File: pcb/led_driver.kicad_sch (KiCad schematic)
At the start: 69 parts, among them J1 48V IN, J2 LED, J3 12V IN, J4 INTERLOCK, Q1 STP30NF10, SW3 ARM, U1 MIC4427, U2 74HC74, U3 74HC08, U4 LM393, U5 L7805

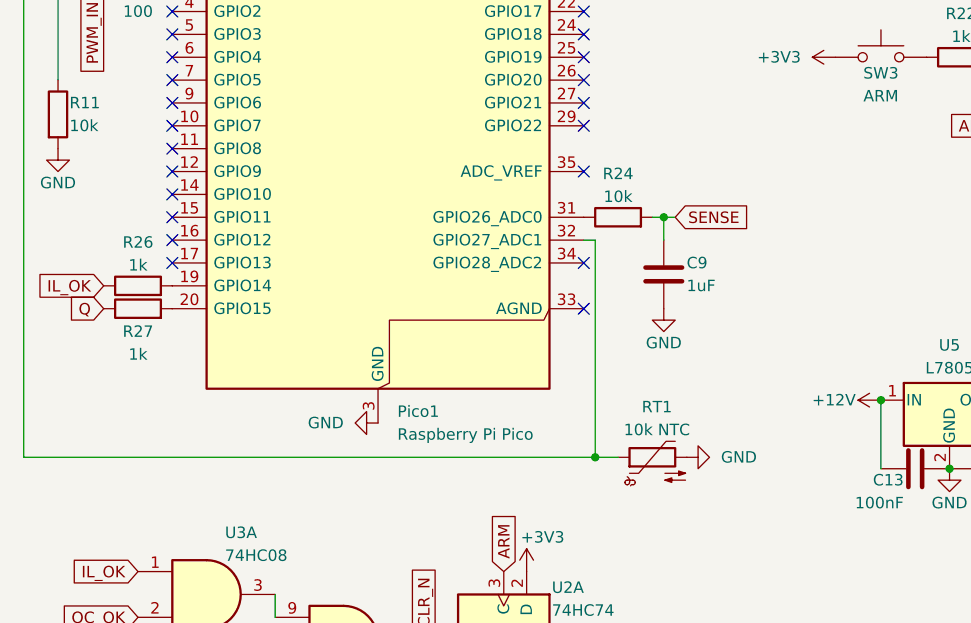
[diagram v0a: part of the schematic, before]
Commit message: First revision
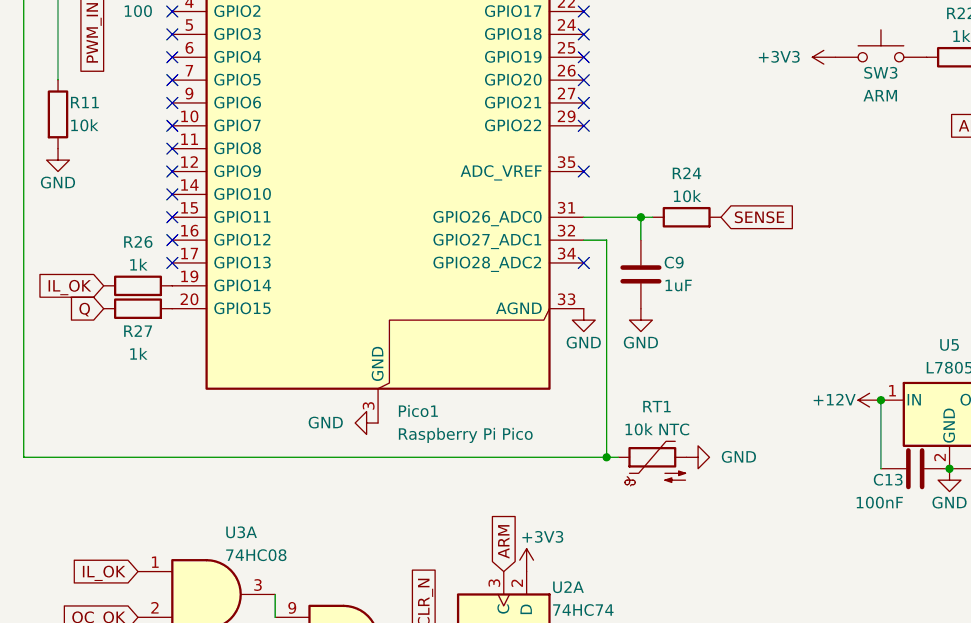
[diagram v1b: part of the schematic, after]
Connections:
- net GND: now also Pico1.33 (AGND)
- net SENSE: no longer C9.1
- net at Pico1.31 (GPIO26_ADC0), R24.1: now also C9.1
- no-connect marks 29 -> 28
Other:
- moved on the sheet: C9, R24
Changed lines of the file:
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@@
 		(title "Fast-Switching LED Driver")
 		(date "2026-09-28")
-		(rev "0")
+		(rev "1")
 	)
 	(text "R2\n4 x 0.39"
@@
 	)
 	(junction
-		(at 111.76 83.82)
+		(at 109.22 83.82)
 		(diameter 0)
 		(color 0 0 0 0)
@@
 	)
 	(junction
-		(at 104.14 110.49)
+		(at 105.41 110.49)
 		(diameter 0)
 		(color 0 0 0 0)
@@
 	)
 	(no_connect
-		(at 102.87 93.98)
-	)
-	(no_connect
 		(at 57.15 81.28)
 	)
@@
 	(wire
 		(pts
-			(xy 102.87 86.36) (xy 104.14 86.36)
+			(xy 102.87 86.36) (xy 105.41 86.36)
 		)
 		(stroke
@@
 	(wire
 		(pts
+			(xy 109.22 83.82) (xy 109.22 86.36)
+		)
+		(stroke
+			(width 0)
+			(type default)
+		)
+	)
+	(wire
+		(pts
 			(xy 203.2 66.04) (xy 199.39 66.04)
 		)
@@
 	(wire
 		(pts
-			(xy 104.14 86.36) (xy 104.14 110.49)
+			(xy 105.41 86.36) (xy 105.41 110.49)
 		)
 		(stroke
@@
 	(wire
 		(pts
-			(xy 111.76 86.36) (xy 111.76 83.82)
-		)
-		(stroke
-			(width 0)
-			(type default)
-		)
-	)
-	(wire
-		(pts
 			(xy 231.14 31.75) (xy 236.22 31.75)
 		)
@@
 	(wire
 		(pts
-			(xy 104.14 110.49) (xy 106.68 110.49)
-		)
-		(stroke
-			(width 0)
-			(type default)
-		)
-	)
-	(wire
-		(pts
 			(xy 57.15 21.59) (xy 85.09 21.59)
 		)
@@
 	(wire
 		(pts
-			(xy 113.03 83.82) (xy 111.76 83.82)
-		)
-		(stroke
-			(width 0)
-			(type default)
-		)
-	)
-	(wire
-		(pts
 			(xy 207.01 137.16) (xy 217.17 137.16)
 		)
@@
 	(wire
 		(pts
-			(xy 111.76 83.82) (xy 110.49 83.82)
+			(xy 229.87 36.83) (xy 231.14 36.83)
 		)
 		(stroke
@@
 	(wire
 		(pts
-			(xy 229.87 36.83) (xy 231.14 36.83)
+			(xy 85.09 21.59) (xy 85.09 33.02)
 		)
 		(stroke
@@
 	(wire
 		(pts
-			(xy 85.09 21.59) (xy 85.09 33.02)
+			(xy 40.64 21.59) (xy 40.64 110.49)
 		)
 		(stroke
@@
 	(wire
 		(pts
-			(xy 40.64 21.59) (xy 40.64 110.49)
+			(xy 40.64 110.49) (xy 106.68 110.49)
 		)
 		(stroke
@@
 	(wire
 		(pts
-			(xy 40.64 110.49) (xy 104.14 110.49)
+			(xy 243.84 66.04) (xy 243.84 57.15)
 		)
 		(stroke
@@
 	(wire
 		(pts
-			(xy 243.84 66.04) (xy 243.84 57.15)
+			(xy 148.59 46.99) (xy 151.13 46.99)
 		)
 		(stroke
@@
 	(wire
 		(pts
-			(xy 148.59 46.99) (xy 151.13 46.99)
+			(xy 199.39 36.83) (xy 196.85 36.83)
 		)
 		(stroke
@@
 	(wire
 		(pts
-			(xy 199.39 36.83) (xy 196.85 36.83)
+			(xy 195.58 137.16) (xy 200.66 137.16)
 		)
 		(stroke
@@
 	(wire
 		(pts
-			(xy 195.58 137.16) (xy 200.66 137.16)
+			(xy 102.87 83.82) (xy 110.49 83.82)
 		)
 		(stroke
@@
 	(global_label "SENSE"
 		(shape input)
-		(at 113.03 83.82 0)
+		(at 118.11 83.82 0)
 		(fields_autoplaced yes)
 		(effects
@@
 		)
 		(property "Intersheetrefs" "${INTERSHEET_REFS}"
-			(at 122.0627 83.82 0)
+			(at 127.1427 83.82 0)
 			(hide yes)
 			(show_name no)
@@
 	(symbol
 		(lib_id "Device:C")
-		(at 111.76 90.17 0)
+		(at 109.22 90.17 0)
 		(unit 1)
 		(body_style 1)
@@
 		(dnp no)
 		(property "Reference" "C9"
-			(at 114.3 88.9 0)
+			(at 111.76 88.9 0)
 			(show_name no)
 			(do_not_autoplace no)
@@
 		)
 		(property "Value" "1uF"
-			(at 114.3 91.44 0)
+			(at 111.76 91.44 0)
 			(show_name no)
 			(do_not_autoplace no)
@@
 		)
 		(property "Footprint" "Capacitor_THT:C_Rect_L7.2mm_W4.5mm_P5.00mm_FKS2_FKP2_MKS2_MKP2"
-			(at 112.7252 93.98 0)
+			(at 110.1852 93.98 0)
 			(hide yes)
 			(show_name no)
@@
 		)
 		(property "Datasheet" ""
-			(at 111.76 90.17 0)
+			(at 109.22 90.17 0)
 			(hide yes)
 			(show_name no)
@@
 		)
 		(property "Description" "Unpolarized capacitor"
-			(at 111.76 90.17 0)
+			(at 109.22 90.17 0)
 			(hide yes)
 			(show_name no)
@@
 	(symbol
 		(lib_id "Device:R")
-		(at 106.68 83.82 90)
+		(at 114.3 83.82 90)
 		(unit 1)
 		(body_style 1)
@@
 		(dnp no)
 		(property "Reference" "R24"
-			(at 106.68 78.994 90)
+			(at 114.3 78.994 90)
 			(show_name no)
 			(do_not_autoplace no)
@@
 		)
 		(property "Value" "10k"
-			(at 106.68 81.534 90)
+			(at 114.3 81.534 90)
 			(show_name no)
 			(do_not_autoplace no)
@@
 		)
 		(property "Footprint" "Resistor_THT:R_Axial_DIN0207_L6.3mm_D2.5mm_P10.16mm_Horizontal"
-			(at 106.68 85.598 90)
+			(at 114.3 85.598 90)
 			(hide yes)
 			(show_name no)
@@
 		)
 		(property "Datasheet" ""
-			(at 106.68 83.82 0)
+			(at 114.3 83.82 0)
 			(hide yes)
 			(show_name no)
@@
 		)
 		(property "Description" "Resistor"
-			(at 106.68 83.82 0)
+			(at 114.3 83.82 0)
 			(hide yes)
 			(show_name no)
@@
 	)
 	(symbol
+		(lib_id "power:GND")
+		(at 102.87 93.98 0)
+		(unit 1)
+		(body_style 1)
+		(exclude_from_sim no)
+		(in_bom yes)
+		(on_board yes)
+		(in_pos_files yes)
+		(dnp no)
+		(property "Reference" "#PWR035"
+			(at 102.87 100.33 0)
+			(hide yes)
+			(show_name no)
+			(do_not_autoplace no)
+			(effects
+				(font
+					(size 1.27 1.27)
+				)
+			)
+		)
+		(property "Value" "GND"
+			(at 102.87 97.79 0)
+			(show_name no)
+			(do_not_autoplace no)
+			(effects
+				(font
+					(size 1.27 1.27)
+				)
+			)
+		)
+		(property "Footprint" ""
+			(at 102.87 93.98 0)
+			(hide yes)
+			(show_name no)
+			(do_not_autoplace no)
+			(effects
+				(font
+					(size 1.27 1.27)
+				)
+			)
+		)
+		(property "Datasheet" ""
+			(at 102.87 93.98 0)
+			(hide yes)
+			(show_name no)
+			(do_not_autoplace no)
+			(effects
+				(font
+					(size 1.27 1.27)
+				)
+			)
+		)
+		(property "Description" "Power symbol creates a global label with name \"GND\" , ground"
+			(at 102.87 93.98 0)
+			(hide yes)
+			(show_name no)
+			(do_not_autoplace no)
+			(effects
+				(font
+					(size 1.27 1.27)
+				)
+			)
+		)
+		(pin "1"
+		)
+		(instances
+			(project "led_driver"
+				(path "/517fb8ba-efa2-4ff9-8737-3053492b2e56"
+					(reference "#PWR035")
+					(unit 1)
+				)
+			)
+		)
+	)
+	(symbol
 		(lib_id "Connector:Screw_Terminal_01x02")
 		(at 259.08 152.4 270)
@@
 	(symbol
 		(lib_id "power:GND")
-		(at 111.76 93.98 0)
+		(at 109.22 93.98 0)
 		(unit 1)
 		(body_style 1)
@@
 		(dnp no)
 		(property "Reference" "#PWR023"
-			(at 111.76 100.33 0)
+			(at 109.22 100.33 0)
 			(hide yes)
 			(show_name no)
@@
 		)
 		(property "Value" "GND"
-			(at 111.76 97.79 0)
+			(at 109.22 97.79 0)
 			(show_name no)
 			(do_not_autoplace no)
@@
 		)
 		(property "Footprint" ""
-			(at 111.76 93.98 0)
+			(at 109.22 93.98 0)
 			(hide yes)
 			(show_name no)
@@
 		)
 		(property "Datasheet" ""
-			(at 111.76 93.98 0)
+			(at 109.22 93.98 0)
 			(hide yes)
 			(show_name no)
@@
 		)
 		(property "Description" "Power symbol creates a global label with name \"GND\" , ground"
-			(at 111.76 93.98 0)
+			(at 109.22 93.98 0)
 			(hide yes)
 			(show_name no)
